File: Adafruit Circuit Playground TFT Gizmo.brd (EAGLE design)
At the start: 53.3 x 53.3 mm, 46 parts, among them IC4 APX803-SAG, Q1 BSS138, U5 PAM8302AASCR

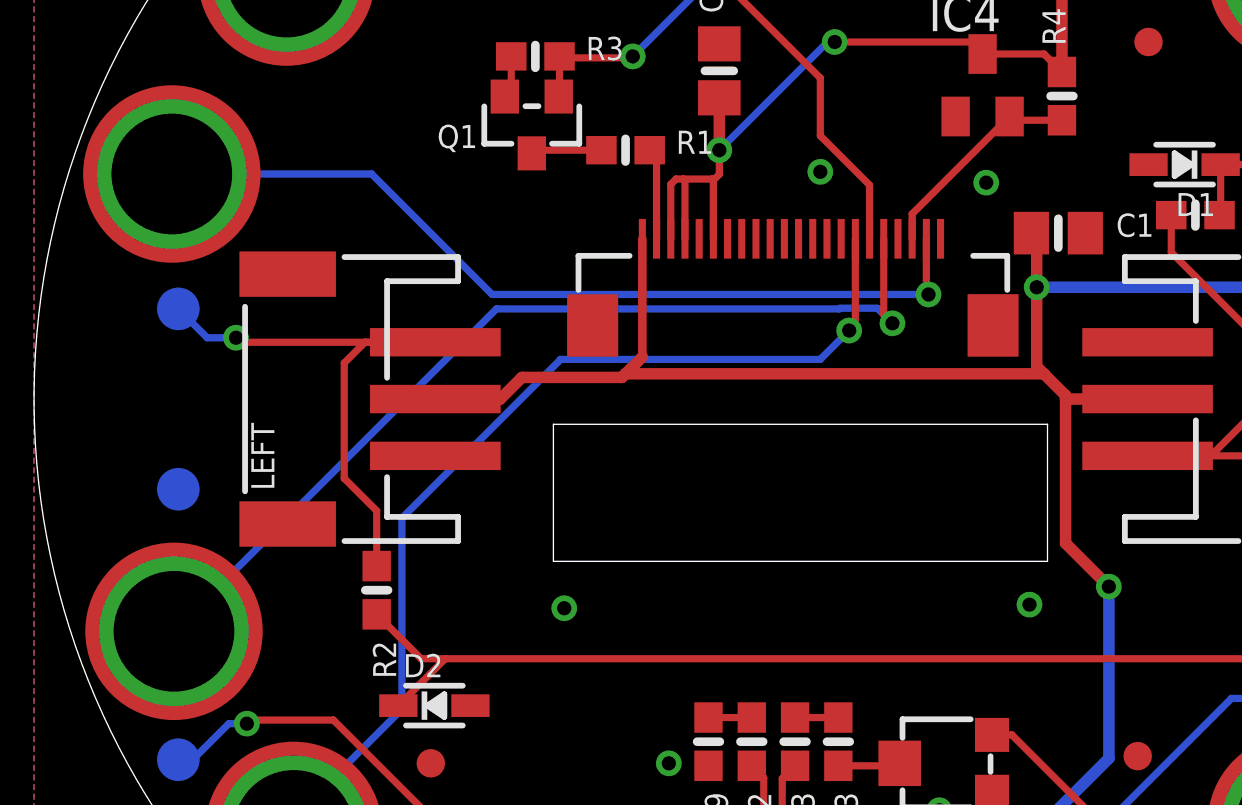
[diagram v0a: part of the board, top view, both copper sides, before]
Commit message: Updated to D1 Revision
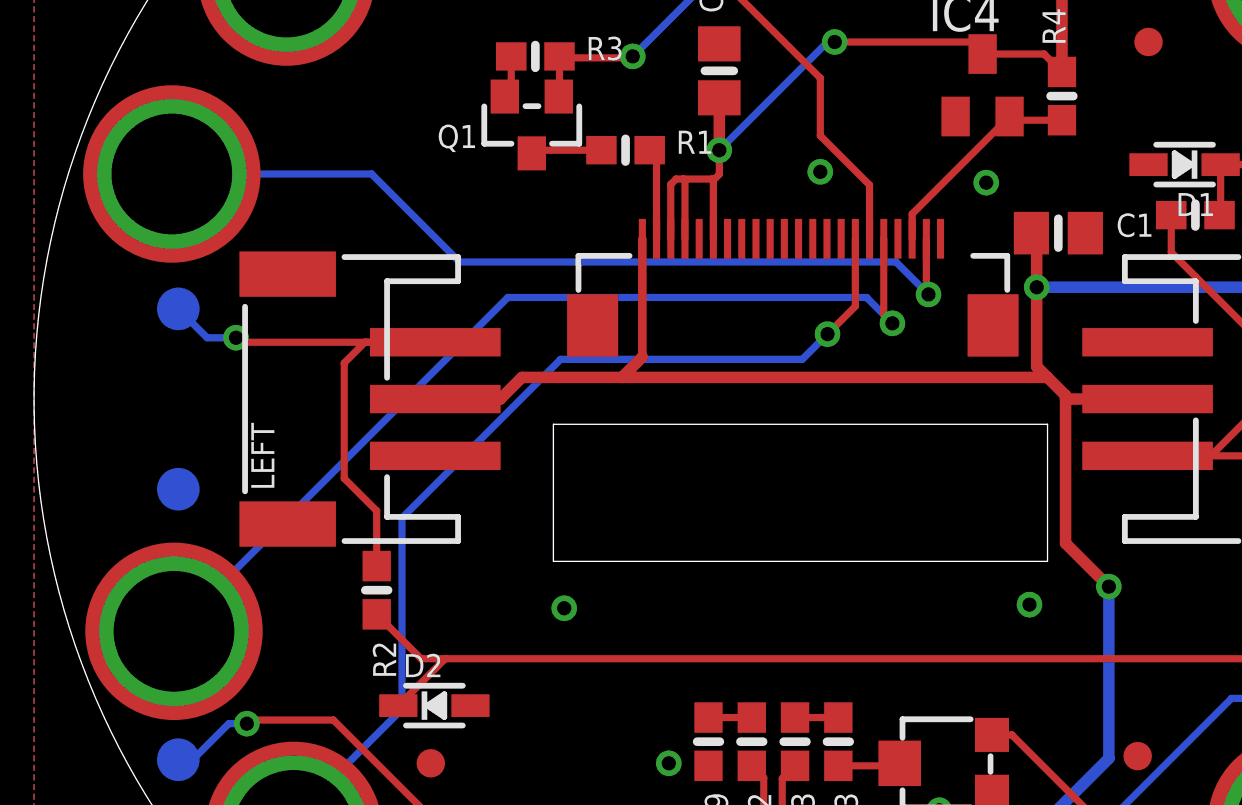
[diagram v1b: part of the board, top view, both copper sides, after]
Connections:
- net A1' renamed A1_
- net A2' renamed A2_
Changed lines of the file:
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@@
 <?xml version="1.0" encoding="utf-8"?>
 <!DOCTYPE eagle SYSTEM "eagle.dtd">
-<eagle version="9.5.1">
+<eagle version="9.5.0">
 <drawing>
 <settings>
@@
 <layer number="45" name="Holes" color="7" fill="1" visible="yes" active="yes"/>
 <layer number="46" name="Milling" color="3" fill="1" visible="yes" active="yes"/>
-<layer number="47" name="Measures" color="7" fill="1" visible="yes" active="yes"/>
+<layer number="47" name="Measures" color="7" fill="1" visible="no" active="yes"/>
 <layer number="48" name="Document" color="7" fill="1" visible="no" active="yes"/>
 <layer number="49" name="Reference" color="7" fill="1" visible="no" active="yes"/>
@@
 <layer number="196" name="mValues" color="7" fill="1" visible="yes" active="yes"/>
 <layer number="199" name="Contour" color="7" fill="1" visible="no" active="yes"/>
-<layer number="200" name="200bmp" color="13" fill="10" visible="yes" active="yes"/>
-<layer number="201" name="201bmp" color="14" fill="1" visible="no" active="yes"/>
+<layer number="200" name="200bmp" color="14" fill="10" visible="yes" active="yes"/>
+<layer number="201" name="201bmp" color="13" fill="1" visible="yes" active="yes"/>
 <layer number="202" name="202bmp" color="3" fill="1" visible="no" active="no"/>
 <layer number="203" name="203bmp" color="14" fill="10" visible="yes" active="yes"/>
@@
 <dimension x1="0" y1="-26.67" x2="0" y2="-13.589" x3="37.592" y3="-20.1295" textsize="1.778" layer="47" dtype="vertical" unit="inch"/>
 <dimension x1="0" y1="13.589" x2="0" y2="26.67" x3="37.592" y3="20.1295" textsize="1.778" layer="47" dtype="vertical" unit="inch"/>
-<dimension x1="-26.67" y1="26.67" x2="-26.67" y2="-26.67" x3="-33.02" y3="0" textsize="1.778" layer="47" dtype="horizontal" unit="inch"/>
-<dimension x1="26.67" y1="26.67" x2="-26.67" y2="26.67" x3="0" y3="33.655" textsize="1.778" layer="47" dtype="horizontal" unit="inch"/>
-<dimension x1="-19.431" y1="4.445" x2="19.431" y2="4.318" x3="0" y3="-32.893" textsize="1.778" layer="47" dtype="horizontal" unit="inch"/>
-<dimension x1="-15.748" y1="-6.604" x2="15.748" y2="-3.556" x3="0" y3="-29.591" textsize="1.778" layer="47" dtype="horizontal" unit="inch"/>
-<dimension x1="-5.969" y1="15.748" x2="-5.207" y2="-18.923" x3="32.893" y3="-1.5875" textsize="1.778" layer="47" dtype="vertical" unit="inch"/>
 </plain>
 <attributes>
@@
 <wire x1="-12.54" y1="0" x2="-10.254" y2="0" width="0.4064" layer="1"/>
 <wire x1="-10.254" y1="0" x2="-9.492" y2="0.762" width="0.4064" layer="1"/>
-<wire x1="-5.842" y1="0.889" x2="8.89" y2="0.889" width="0.4064" layer="1"/>
+<wire x1="-5.969" y1="0.762" x2="9.017" y2="0.762" width="0.4064" layer="1"/>
 <wire x1="-9.492" y1="0.762" x2="-5.969" y2="0.762" width="0.4064" layer="1"/>
 <wire x1="-5.25" y1="5.643" x2="-5.25" y2="1.481" width="0.3048" layer="1"/>
-<wire x1="-5.25" y1="1.481" x2="-5.842" y2="0.889" width="0.4064" layer="1"/>
-<wire x1="-5.842" y1="0.889" x2="-5.969" y2="0.762" width="0.4064" layer="1"/>
+<wire x1="-5.25" y1="1.481" x2="-5.969" y2="0.762" width="0.4064" layer="1"/>
 <wire x1="3.175" y1="-16.195" x2="2.052" y2="-15.072" width="0.4064" layer="1"/>
 <wire x1="2.052" y1="-15.072" x2="0.975" y2="-15.072" width="0.4064" layer="1"/>
@@
 <wire x1="8.636" y1="3.937" x2="8.636" y2="1.143" width="0.4064" layer="1"/>
 <wire x1="9.652" y1="0" x2="9.652" y2="0.127" width="0.4064" layer="1"/>
-<wire x1="9.652" y1="0.127" x2="8.89" y2="0.889" width="0.4064" layer="1"/>
-<wire x1="8.89" y1="0.889" x2="8.636" y2="1.143" width="0.4064" layer="1"/>
+<wire x1="9.652" y1="0.127" x2="9.017" y2="0.762" width="0.4064" layer="1"/>
+<wire x1="9.017" y1="0.762" x2="8.636" y2="1.143" width="0.4064" layer="1"/>
 <contactref element="TP17" pad="P$1"/>
 <via x="8.636" y="3.937" extent="1-16" drill="0.5"/>
@@
 <wire x1="4.75" y1="3.759" x2="4.826" y2="3.683" width="0.254" layer="1"/>
 <via x="4.826" y="3.683" extent="1-16" drill="0.5"/>
-<wire x1="4.826" y1="3.683" x2="-10.541" y2="3.683" width="0.254" layer="16"/>
+<wire x1="4.826" y1="3.683" x2="3.683" y2="4.826" width="0.254" layer="16"/>
+<wire x1="3.683" y1="4.826" x2="-11.684" y2="4.826" width="0.254" layer="16"/>
 <wire x1="-14.7828" y1="7.9248" x2="-21.8186" y2="7.9248" width="0.254" layer="16"/>
-<wire x1="-10.541" y1="3.683" x2="-14.7828" y2="7.9248" width="0.254" layer="16"/>
+<wire x1="-11.684" y1="4.826" x2="-14.7828" y2="7.9248" width="0.254" layer="16"/>
 </signal>
 <signal name="SCK">
@@
 <wire x1="15.113" y1="6.477" x2="15.074" y2="6.477" width="0.254" layer="1"/>
 </signal>
-<signal name="A2'">
+<signal name="A2_">
 <contactref element="RIGHT" pad="3"/>
 <contactref element="R5" pad="1"/>
@@
 <wire x1="17.399" y1="-2.286" x2="20.701" y2="-2.286" width="0.254" layer="16"/>
 </signal>
-<signal name="A1'">
+<signal name="A1_">
 <contactref element="LEFT" pad="3"/>
 <contactref element="R2" pad="1"/>
@@
 <contactref element="TP13" pad="P$1"/>
 <contactref element="TFT2" pad="16"/>
-<wire x1="2.25" y1="5.643" x2="2.25" y2="2.631" width="0.254" layer="1"/>
-<wire x1="2.25" y1="2.631" x2="2.032" y2="2.413" width="0.254" layer="1"/>
-<via x="2.032" y="2.413" extent="1-16" drill="0.5"/>
-<wire x1="2.032" y1="2.413" x2="1.016" y2="1.397" width="0.254" layer="16"/>
+<wire x1="2.25" y1="5.643" x2="2.25" y2="3.266" width="0.254" layer="1"/>
+<wire x1="2.25" y1="3.266" x2="1.27" y2="2.286" width="0.254" layer="1"/>
+<via x="1.27" y="2.286" extent="1-16" drill="0.5"/>
+<wire x1="1.27" y1="2.286" x2="0.381" y2="1.397" width="0.254" layer="16"/>
 <wire x1="-13.716" y1="-4.191" x2="-13.716" y2="-10.922" width="0.254" layer="16"/>
 <wire x1="-13.716" y1="-10.922" x2="-17.526" y2="-14.732" width="0.254" layer="16"/>
 <wire x1="-17.526" y1="-14.732" x2="-17.526" y2="-15.1892" width="0.254" layer="16"/>
-<wire x1="1.016" y1="1.397" x2="-8.128" y2="1.397" width="0.254" layer="16"/>
+<wire x1="0.381" y1="1.397" x2="-8.128" y2="1.397" width="0.254" layer="16"/>
 <wire x1="-8.128" y1="1.397" x2="-13.716" y2="-4.191" width="0.254" layer="16"/>
 </signal>
@@
 <wire x1="3.25" y1="2.973" x2="3.556" y2="2.667" width="0.254" layer="1"/>
 <via x="3.556" y="2.667" extent="1-16" drill="0.5"/>
-<wire x1="1.7075" y1="3.1964" x2="1.6861" y2="3.175" width="0.254" layer="16"/>
-<wire x1="3.556" y1="2.667" x2="3.0266" y2="3.1964" width="0.254" layer="16"/>
-<wire x1="3.0266" y1="3.1964" x2="1.7075" y2="3.1964" width="0.254" layer="16"/>
-<wire x1="-10.3886" y1="3.175" x2="-21.7424" y2="-8.1788" width="0.254" layer="16"/>
-<wire x1="1.6861" y1="3.175" x2="-10.3886" y2="3.175" width="0.254" layer="16"/>
+<wire x1="3.556" y1="2.667" x2="2.6456" y2="3.5774" width="0.254" layer="16"/>
+<wire x1="-9.9862" y1="3.5774" x2="-21.7424" y2="-8.1788" width="0.254" layer="16"/>
+<wire x1="2.6456" y1="3.5774" x2="-9.9862" y2="3.5774" width="0.254" layer="16"/>
 </signal>
 <signal name="LEDK">
